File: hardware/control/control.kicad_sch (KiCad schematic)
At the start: 46 parts, among them IC1 TMUX4053DYYR, J0 43045-0412, J1 Conn_01x02_Pin, J11 Conn_01x04_Pin, J12 Camera Isolated triggers (ope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, J2 Conn_01x02_Pin, J3 Conn_01x02_Pin, J4 Conn_01x02_Pin, J5 Conn_01x05_Pin, J6 Conn_01x04_Pin, J7 Screw_Terminal_01x02, J8 Camera Isolated triggers (ope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, U2 MCP4728, U3 MAX6675ISA_, U4 R-78HB12-0.5, U5 R-78HB5.0-0.5

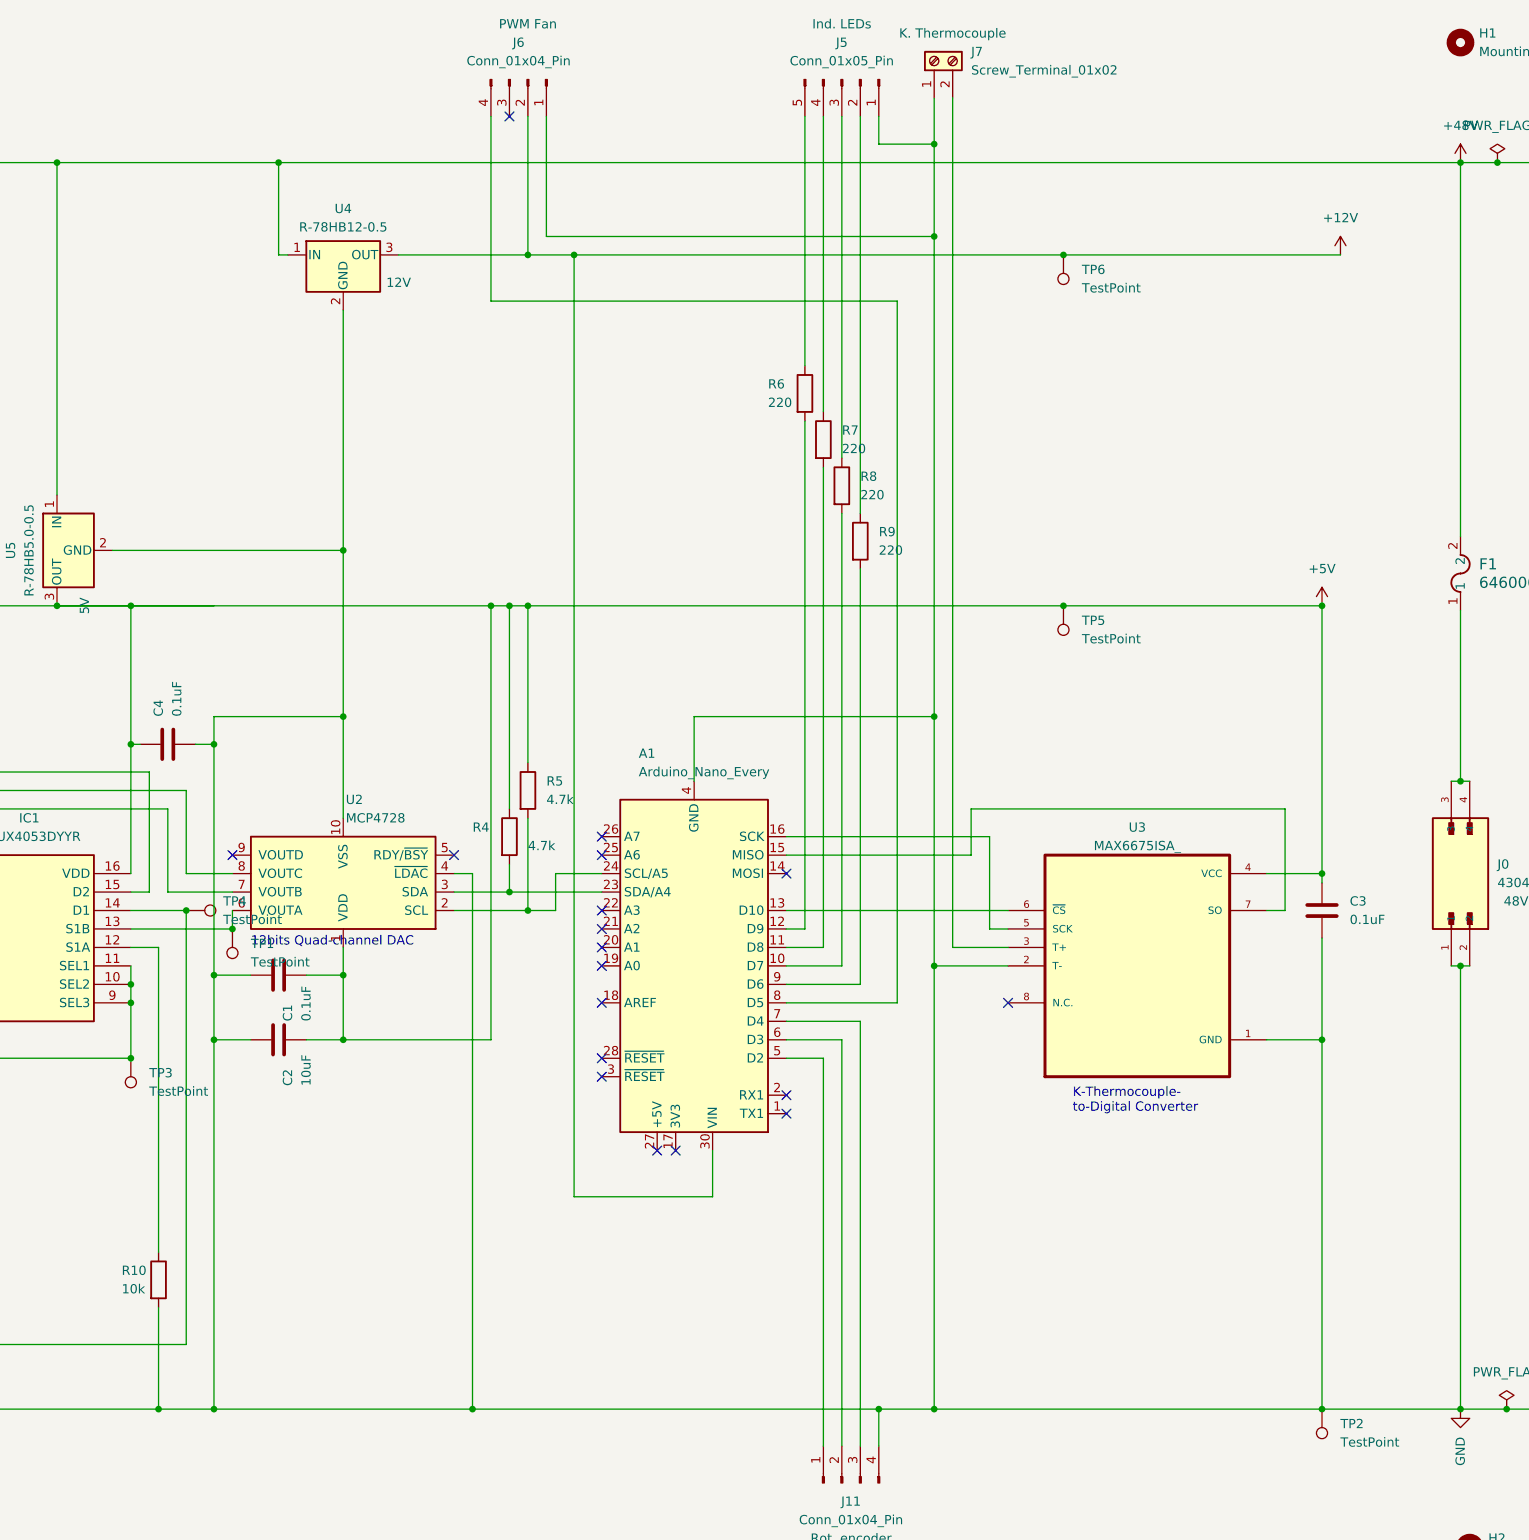
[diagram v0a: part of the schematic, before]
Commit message: removing old thermocouple ic
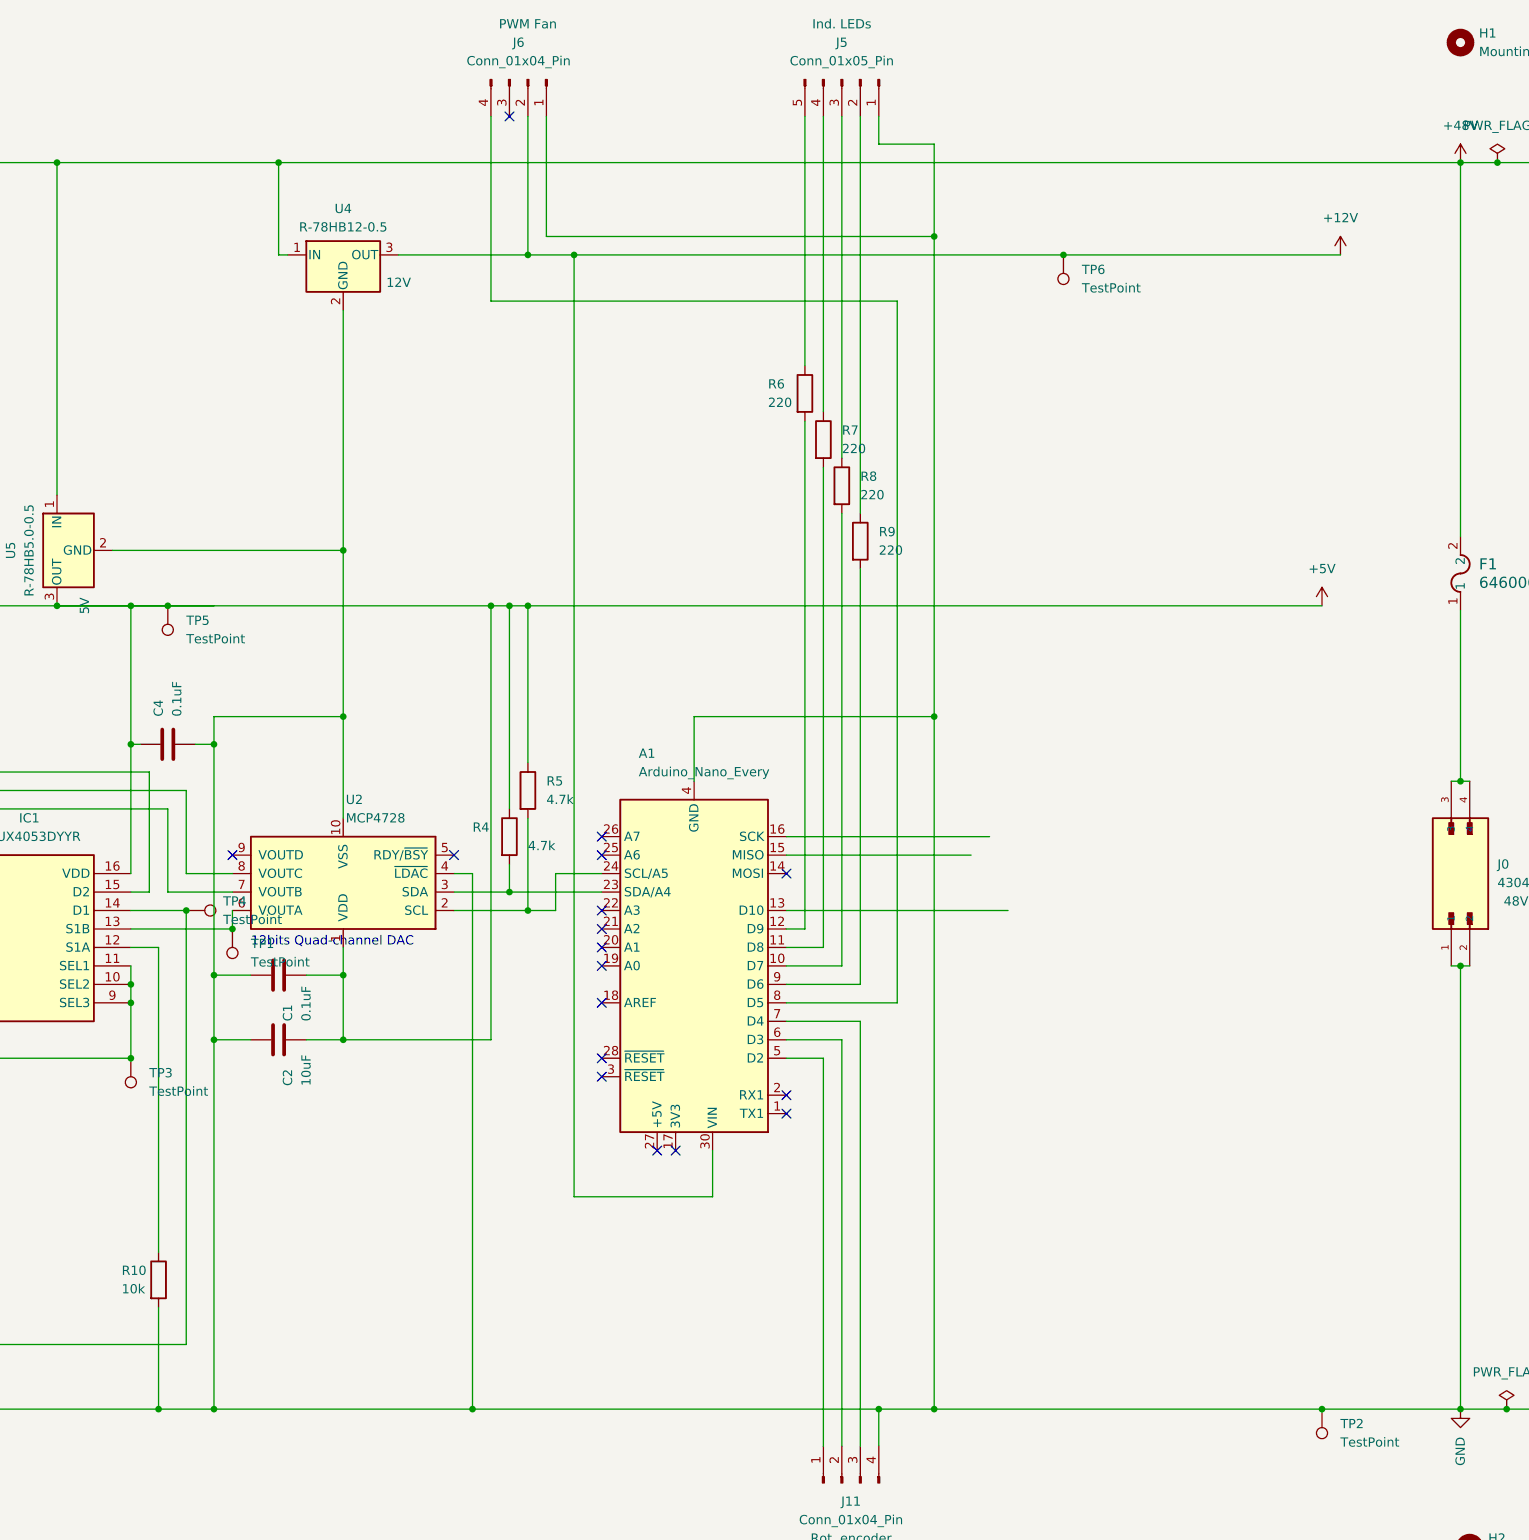
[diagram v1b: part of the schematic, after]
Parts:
- removed C3: 0.1uF, Capacitor_THT:C_Disc_D5.0mm_W2.5mm_P2.50mm, symbol Device:C
- removed J7: Screw_Terminal_01x02, TerminalBlock_Phoenix:TerminalBlock_Phoenix_MKDS-1,5-2_1x02_P5.00mm_Horizontal, symbol Connector:Screw_Terminal_01x02
- removed U3: MAX6675ISA_, MAX6675ISA_:SOIC127P600X175-8N, symbol MAX6675ISA_:MAX6675ISA_
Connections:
- no-connect marks 18 -> 17
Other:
- note removed: "K-Thermocouple- to-Digital Converter"
- moved on the sheet: TP5
